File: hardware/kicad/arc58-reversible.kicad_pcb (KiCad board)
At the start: 2 copper layers, 180 x 160 mm, 91 parts, among them J1 MJ-4PP-9_Reversible, J2 SSD1306 OLED 128x32, SW1 SW_PUSH_LED, SW10 SW_PUSH_LED, SW11 SW_PUSH_LED, SW12 SW_PUSH_LED, SW13 SW_PUSH_LED, SW14 SW_PUSH_LED, SW15 SW_PUSH_LED, SW16 SW_PUSH_LED, SW17 SW_PUSH_LED, SW18 SW_PUSH_LED, SW19 SW_PUSH_LED, SW2 SW_PUSH_LED, SW20 SW_PUSH_LED, SW21 SW_PUSH_LED, SW22 SW_PUSH_LED, SW23 SW_PUSH_LED, SW24 SW_PUSH_LED, SW25 Rotary_Encoder_Switch, SW26 SW_PUSH_LED, SW27 SW_PUSH_LED, SW28 SW_PUSH_LED, SW29 SW_PUSH_LED, SW3 SW_PUSH_LED, SW4 SW_PUSH_LED, SW5 SW_PUSH_LED, SW6 SW_PUSH_LED, SW7 SW_PUSH_LED, SW8 SW_PUSH_LED, SW9 SW_PUSH_LED, U1 KEEBD Helios RP2040, U2 74AHCT1G125

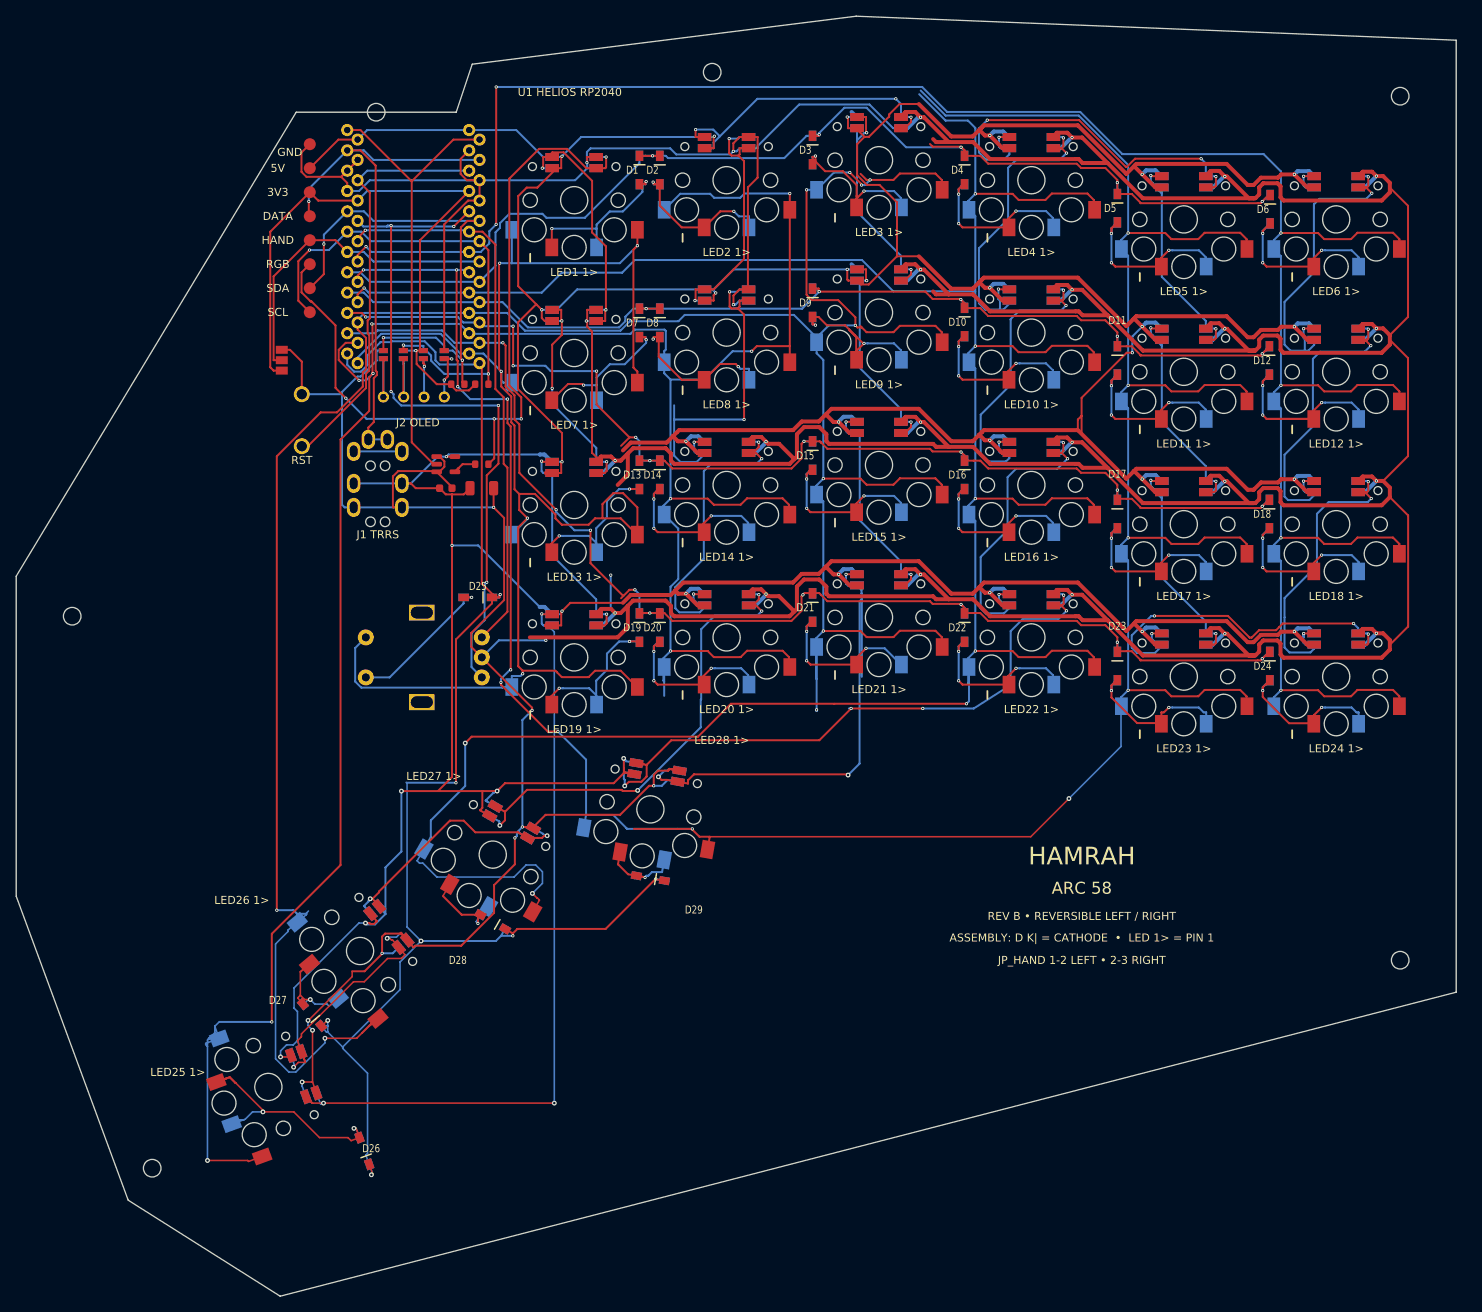
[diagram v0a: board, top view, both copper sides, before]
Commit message: Complete Arc 58 Rev Alpha design
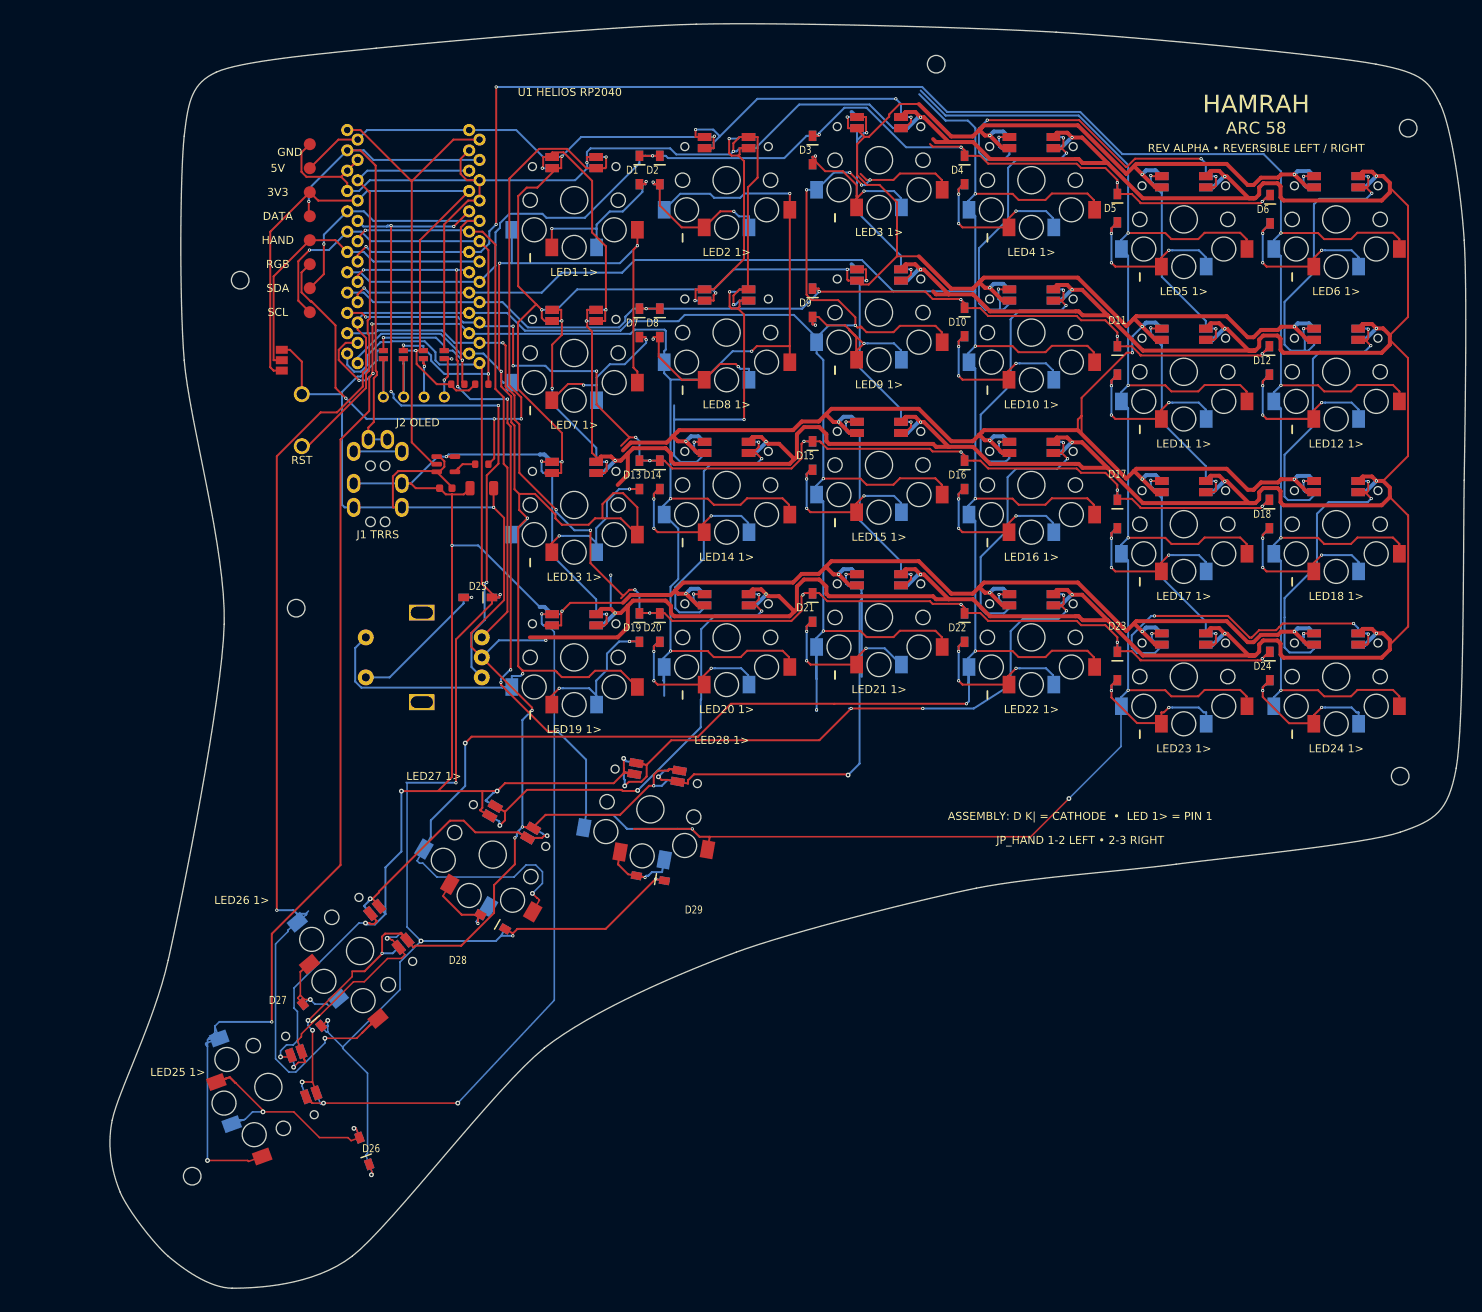
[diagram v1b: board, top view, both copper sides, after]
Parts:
- moved H2 28.0 mm to (165.8, 33.0)
- moved H4 28.0 mm to (85.8, 101.0)
- moved H3 27.0 mm to (78.8, 60.0)
- moved H6 23.0 mm to (223.8, 122.0)
- moved H5 5.10 mm to (72.8, 172.0)
- moved H1 4.12 mm to (224.8, 41.0)
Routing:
- net Net-(SW19-Pad2): track 100.3 -> 93.0 mm
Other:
- board size 180 x 160 mm -> 169.5 x 158.1 mm
- board text added: "REV ALPHA • REVERSIBLE LEFT / RIGHT"
- board text removed: "REV B • REVERSIBLE LEFT / RIGHT"
